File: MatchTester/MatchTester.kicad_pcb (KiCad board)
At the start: 2 copper layers, 85 x 54 mm, 51 parts, among them J1 Conn_01x01, J10 Conn_01x01, J11 Conn_01x01, J12 Conn_01x01, J13 Conn_01x01, J14 Conn_01x01, J2 Conn_Coaxial, J20 Conn_Coaxial, J21 Conn_01x01, J22 Conn_01x01, J25 Conn_01x01, J26 Conn_01x01, J29 Conn_01x01, J3 Conn_Coaxial, J30 Conn_01x01, J31 Conn_01x01, J33 Conn_01x03, J4 Conn_Coaxial, J5 Conn_01x02, J7 Conn_01x01, J8 Conn_01x01, J9 Conn_01x01

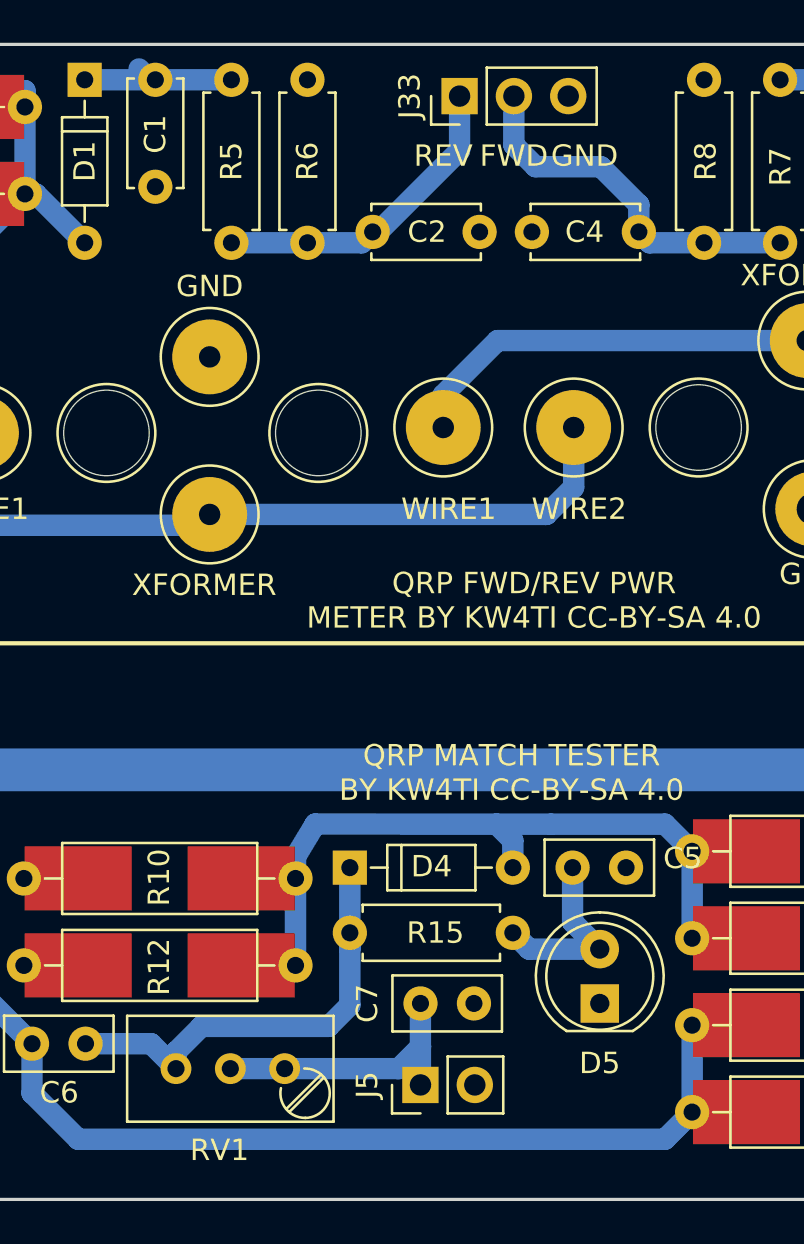
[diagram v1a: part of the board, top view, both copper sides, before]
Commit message: Converted all Kicad projects to version 6.0.10
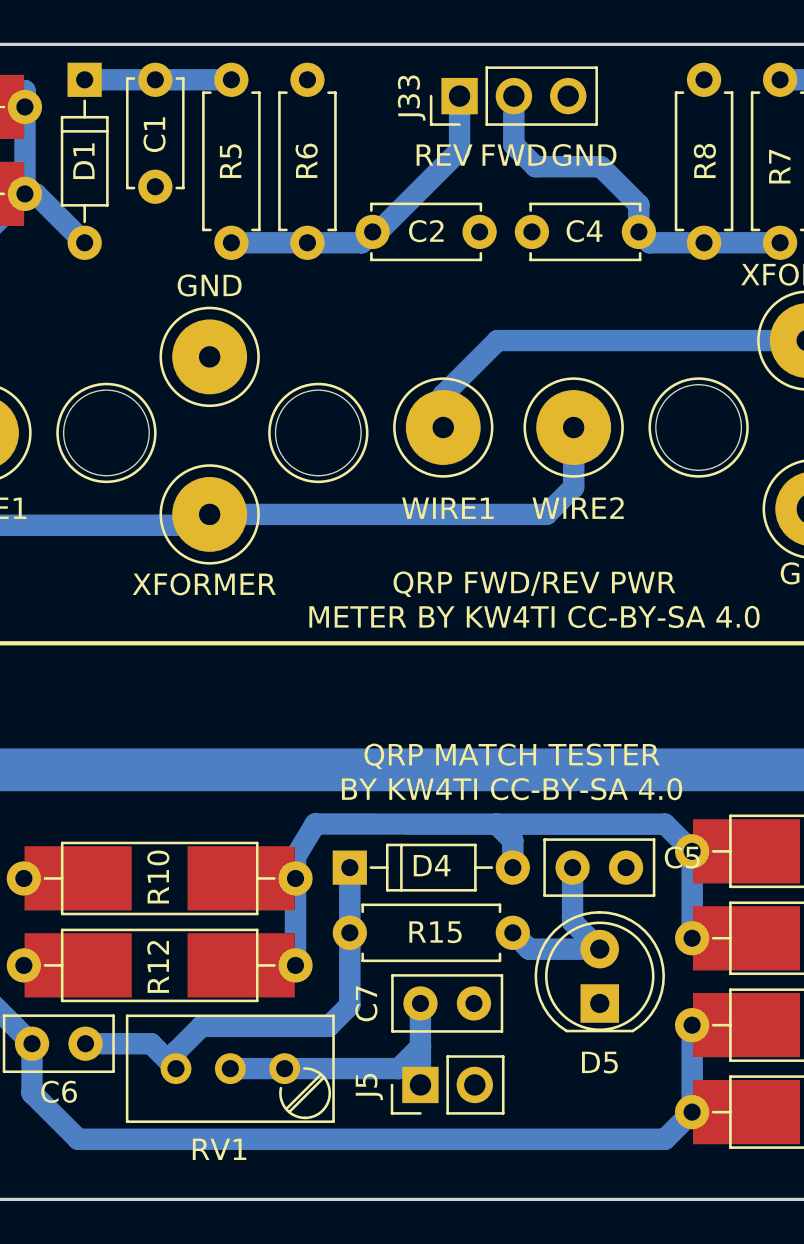
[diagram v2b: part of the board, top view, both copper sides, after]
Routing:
- net Net-(C6-Pad2): track 21.7 -> 21.0 mm
- net Net-(R5-Pad2): track 7.83 -> 7.11 mm
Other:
- net class Default removed
